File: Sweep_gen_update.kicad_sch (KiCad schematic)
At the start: 11 parts, among them J1 Switch, J2 IC6 Jumper, U1 74LS00, U2 74LS42, U3 74LS90

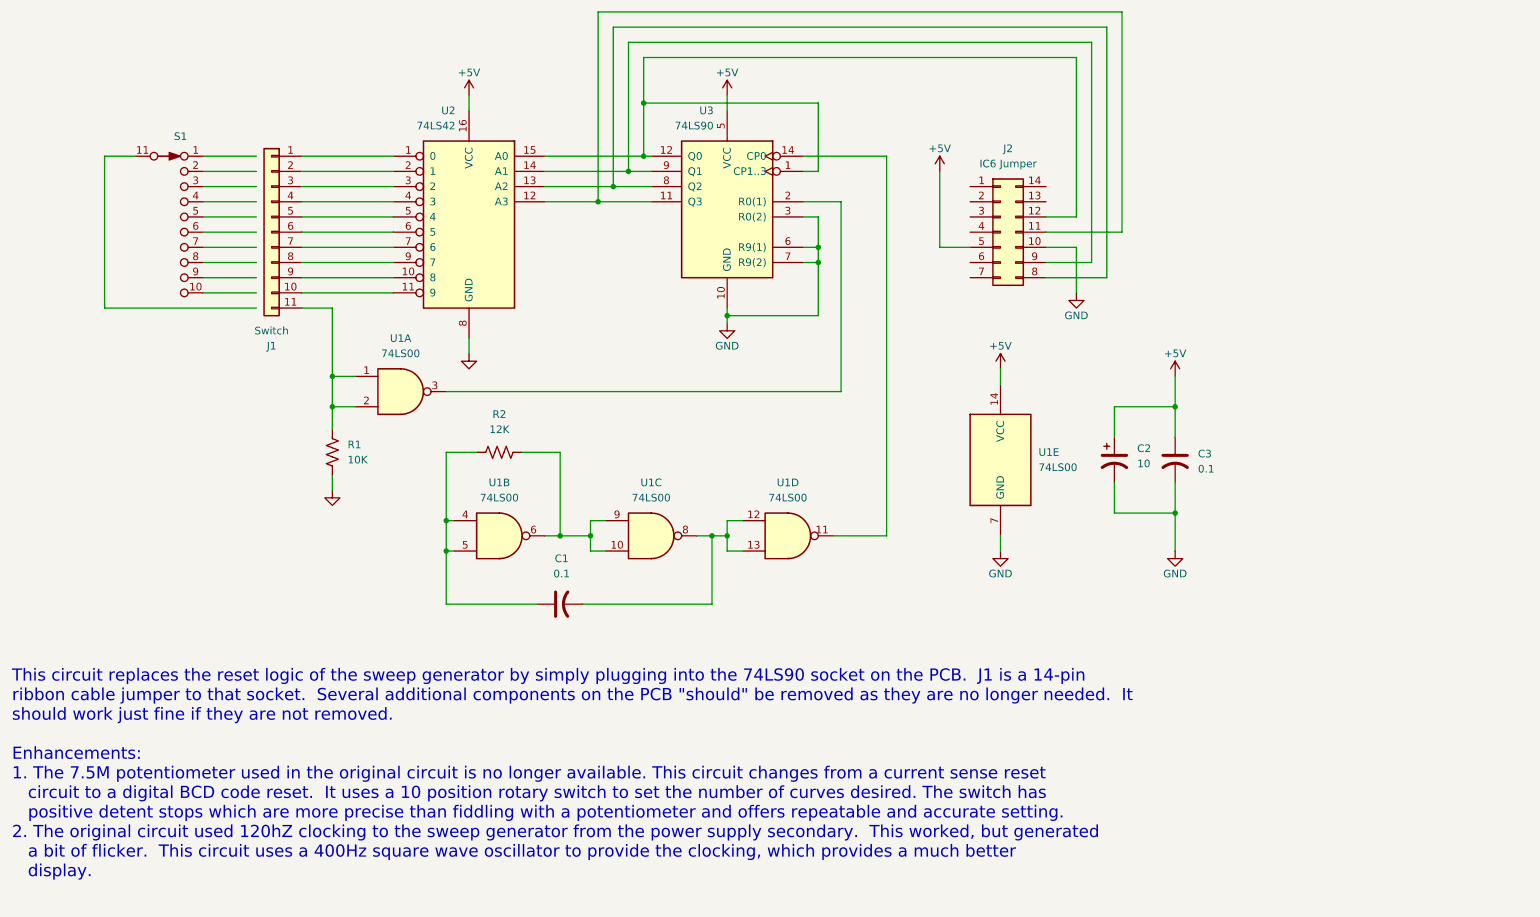
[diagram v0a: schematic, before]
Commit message: testing complete
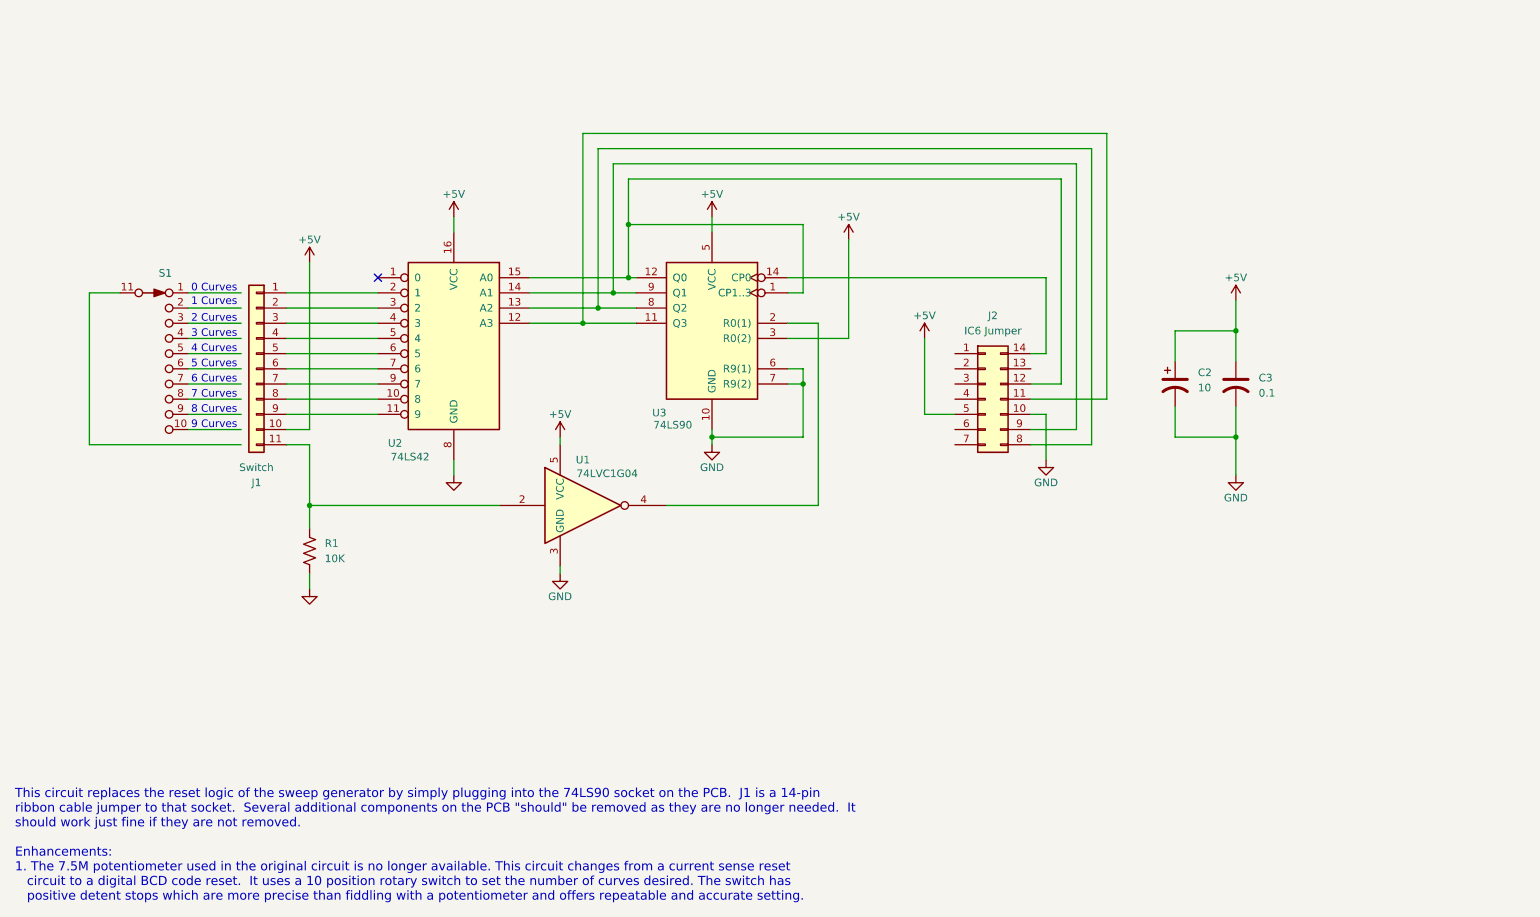
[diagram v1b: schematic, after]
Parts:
- removed C1: 0.1, symbol Device:C_US
- removed R2: 12K, symbol Device:R_US
- removed U1: 74LS00, symbol 74xx:74LS00
- added U1: 74LVC1G04, symbol 74xGxx:74LVC1G04
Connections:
- net +5V: now also J1.10 (Pin_10), U3.3 (R0(2)), U1.5 (VCC)
- net GND: now also U1.3 (GND); no longer U3.3 (R0(2))
- net at J1.11 (Pin_11), R1.1: now also U1.2
- net at U3.2 (R0(1)): now also U1.4
- net at U3.14 (CP0): now also J2.14 (Pin_14)
- net at J1.1 (Pin_1): now also U2.2 (1); no longer U2.1 (0)
- net at U2.11 (9): now also J1.9 (Pin_9); no longer J1.10 (Pin_10)
- net at J1.2 (Pin_2): now also U2.3 (2); no longer U2.2 (1)
- net at J1.3 (Pin_3): now also U2.4 (3); no longer U2.3 (2)
- net at J1.4 (Pin_4): now also U2.5 (4); no longer U2.4 (3)
- net at J1.5 (Pin_5): now also U2.6 (5); no longer U2.5 (4)
- net at J1.6 (Pin_6): now also U2.7 (6); no longer U2.6 (5)
- net at J1.7 (Pin_7): now also U2.9 (7); no longer U2.7 (6)
- net at J1.8 (Pin_8): now also U2.10 (8); no longer U2.9 (7)
- no-connect marks 0 -> 1
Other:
- note added: "0 Curves"
- note added: "1 Curves"
- note added: "2 Curves"
- note added: "3 Curves"
- note added: "4 Curves"
- note added: "5 Curves"
- note added: "6 Curves"
- note added: "7 Curves"
- note added: "8 Curves"
- note added: "9 Curves"
- moved on the sheet: C2, C3, J1, J2, R1, S1, U2, U3
